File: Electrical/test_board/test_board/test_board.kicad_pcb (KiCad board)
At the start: 2 copper layers, 57.5 x 176 mm, 45 parts, among them J1 Conn_01x03_Pin, J10 Conn_01x03_Pin, J10 Conn_01x04_Socket, J11 Conn_01x04_Socket, J12 Conn_01x03_Pin, J14 Conn_01x03_Pin, J2 Screw_Terminal_01x04, J3 Conn_01x04_Socket, J4 Conn_01x04_Socket, J5 Conn_01x04_Socket, J6 Conn_01x03_Pin, J8 Conn_01x03_Pin, J9 Conn_01x04_Socket

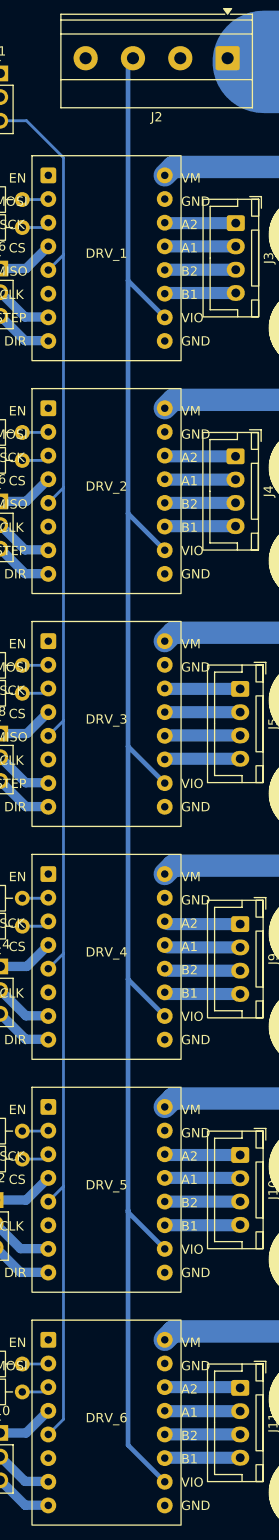
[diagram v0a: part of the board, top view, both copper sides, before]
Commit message: Optical adjustments
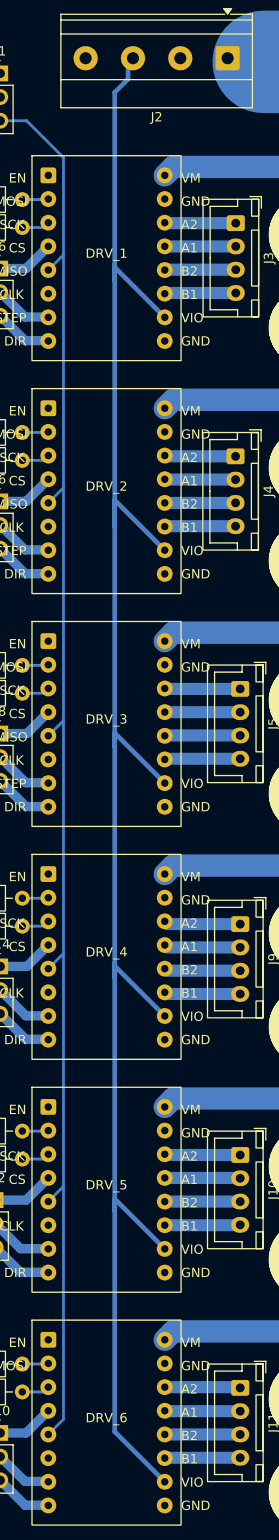
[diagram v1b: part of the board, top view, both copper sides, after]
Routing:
- net +3.3V: track 182.9 -> 203.3 mm
